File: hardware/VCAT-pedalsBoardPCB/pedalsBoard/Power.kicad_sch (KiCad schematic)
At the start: 8 parts

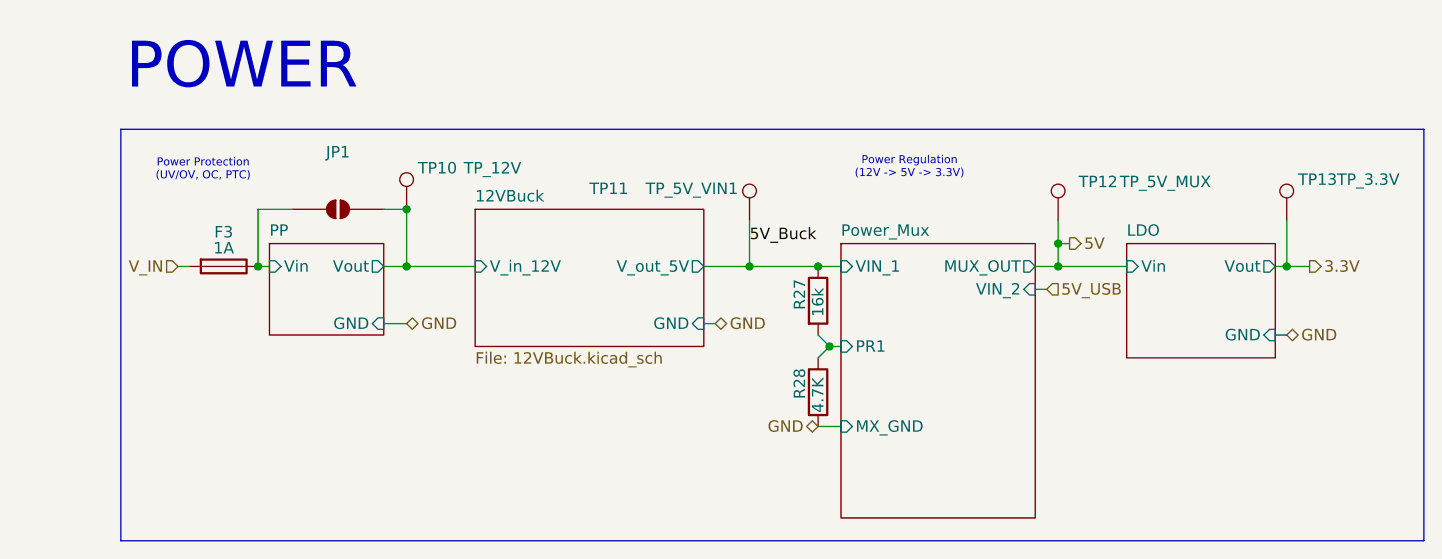
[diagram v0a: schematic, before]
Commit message: tweaked some power labels
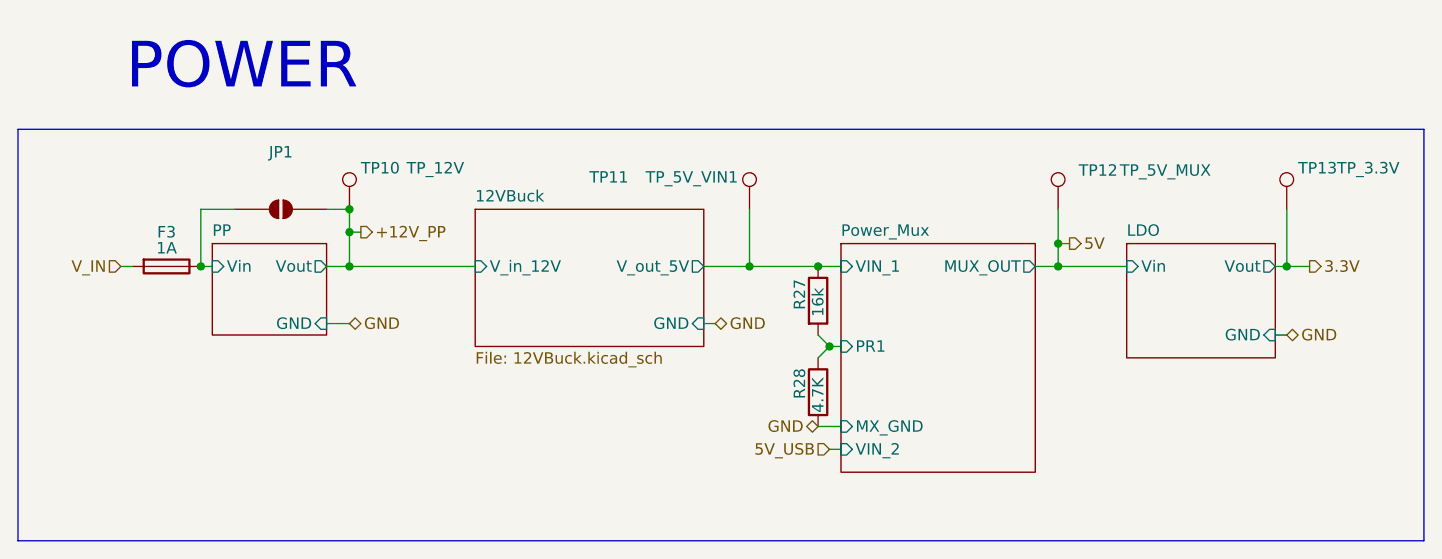
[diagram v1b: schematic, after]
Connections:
- net 12VBuck/V_in_12V renamed +12V_PP
- net 5V_Buck renamed 12VBuck/V_out_5V
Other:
- note removed: "Power Protection (UV/OV, OC, PTC)"
- note removed: "Power Regulation (12V -> 5V -> 3.3V)"
- moved on the sheet: F3, JP1, TP10, TP11, TP12, TP13
